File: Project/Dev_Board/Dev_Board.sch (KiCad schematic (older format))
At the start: 1 part

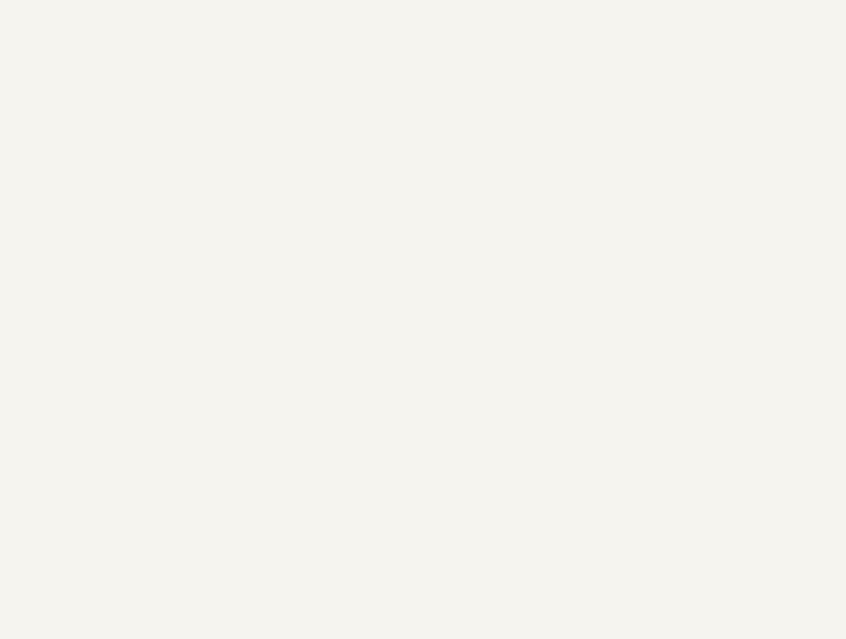
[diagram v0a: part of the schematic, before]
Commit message: with headers
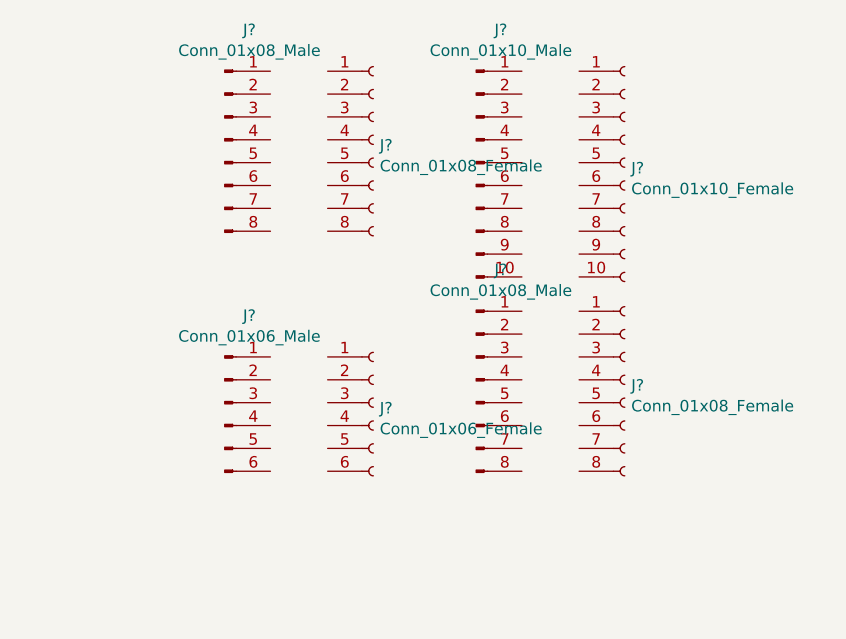
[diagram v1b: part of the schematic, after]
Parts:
- added J? (x2): Conn_01x08_Male, symbol Connector:Conn_01x08_Male
- added J? (x2): Conn_01x08_Female, symbol Connector:Conn_01x08_Female
- added J?: Conn_01x06_Female, symbol Connector:Conn_01x06_Female
- added J?: Conn_01x06_Male, symbol Connector:Conn_01x06_Male
- added J?: Conn_01x10_Male, symbol Connector:Conn_01x10_Male
- added J?: Conn_01x10_Female, symbol Connector:Conn_01x10_Female
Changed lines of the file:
@@
+	1    0    0    -1
+$EndComp
+$Comp
+L Connector:Conn_01x06_Female J?
+U 1 1 5CF178B3
+P 9950 2150
+F 0 "J?" H 9978 2126 50  0000 L CNN
+F 1 "Conn_01x06_Female" H 9978 2035 50  0000 L CNN
+F 2 "" H 9950 2150 50  0001 C CNN
+F 3 "~" H 9950 2150 50  0001 C CNN
+	1    9950 2150
+	1    0    0    -1
+$EndComp
+$Comp
+L Connector:Conn_01x06_Male J?
+U 1 1 5CF18C99
+P 9300 2150
+F 0 "J?" H 9408 2531 50  0000 C CNN
+F 1 "Conn_01x06_Male" H 9408 2440 50  0000 C CNN
+F 2 "" H 9300 2150 50  0001 C CNN
+F 3 "~" H 9300 2150 50  0001 C CNN
+	1    9300 2150
+	1    0    0    -1
+$EndComp
+$Comp
+L Connector:Conn_01x08_Female J?
+U 1 1 5CF16C3E
+P 9950 1000
+F 0 "J?" H 9978 976 50  0000 L CNN
+F 1 "Conn_01x08_Female" H 9978 885 50  0000 L CNN
+F 2 "" H 9950 1000 50  0001 C CNN
+F 3 "~" H 9950 1000 50  0001 C CNN
+	1    9950 1000
+	1    0    0    -1
+$EndComp
+$Comp
+L Connector:Conn_01x08_Male J?
+U 1 1 5CF15183
+P 9300 1000
+F 0 "J?" H 9408 1481 50  0000 C CNN
+F 1 "Conn_01x08_Male" H 9408 1390 50  0000 C CNN
+F 2 "" H 9300 1000 50  0001 C CNN
+F 3 "~" H 9300 1000 50  0001 C CNN
+	1    9300 1000
+	1    0    0    -1
+$EndComp
+$Comp
+L Connector:Conn_01x08_Female J?
+U 1 1 5CF23AB4
+P 11050 2050
+F 0 "J?" H 11078 2026 50  0000 L CNN
+F 1 "Conn_01x08_Female" H 11078 1935 50  0000 L CNN
+F 2 "" H 11050 2050 50  0001 C CNN
+F 3 "~" H 11050 2050 50  0001 C CNN
+	1    11050 2050
+	1    0    0    -1
+$EndComp
+$Comp
+L Connector:Conn_01x08_Male J?
+U 1 1 5CF23ABA
+P 10400 2050
+F 0 "J?" H 10508 2531 50  0000 C CNN
+F 1 "Conn_01x08_Male" H 10508 2440 50  0000 C CNN
+F 2 "" H 10400 2050 50  0001 C CNN
+F 3 "~" H 10400 2050 50  0001 C CNN
+	1    10400 2050
+	1    0    0    -1
+$EndComp
+$Comp
+L Connector:Conn_01x10_Male J?
+U 1 1 5CF24CE7
+P 10400 1100
+F 0 "J?" H 10508 1681 50  0000 C CNN
+F 1 "Conn_01x10_Male" H 10508 1590 50  0000 C CNN
+F 2 "" H 10400 1100 50  0001 C CNN
+F 3 "~" H 10400 1100 50  0001 C CNN
+	1    10400 1100
+	1    0    0    -1
+$EndComp
+$Comp
+L Connector:Conn_01x10_Female J?
+U 1 1 5CF26CEC
+P 11050 1100
+F 0 "J?" H 11078 1076 50  0000 L CNN
+F 1 "Conn_01x10_Female" H 11078 985 50  0000 L CNN
+F 2 "" H 11050 1100 50  0001 C CNN
+F 3 "~" H 11050 1100 50  0001 C CNN
+	1    11050 1100
 	1    0    0    -1
 $EndComp
